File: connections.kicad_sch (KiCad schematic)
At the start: 27 parts, among them J1 Conn_01x04_Pin, J2 Conn_02x07_Odd_Even, J3 Conn_01x01_Pin, Q1 BSS138, Q2 BSS138

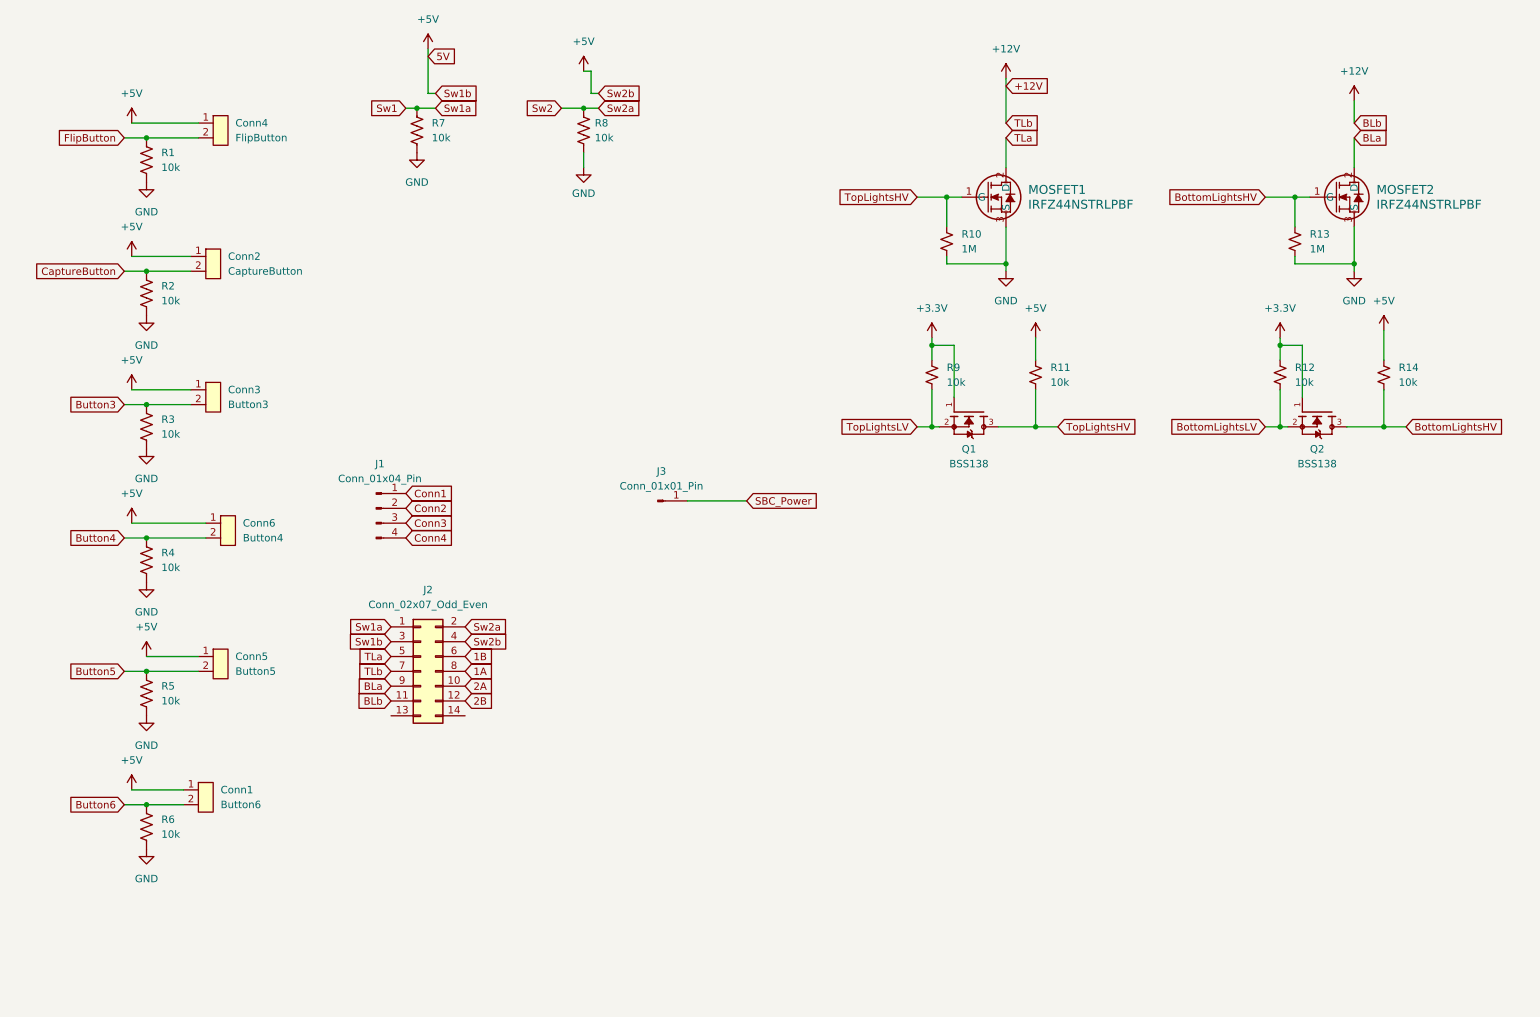
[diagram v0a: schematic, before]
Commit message: Layout changes
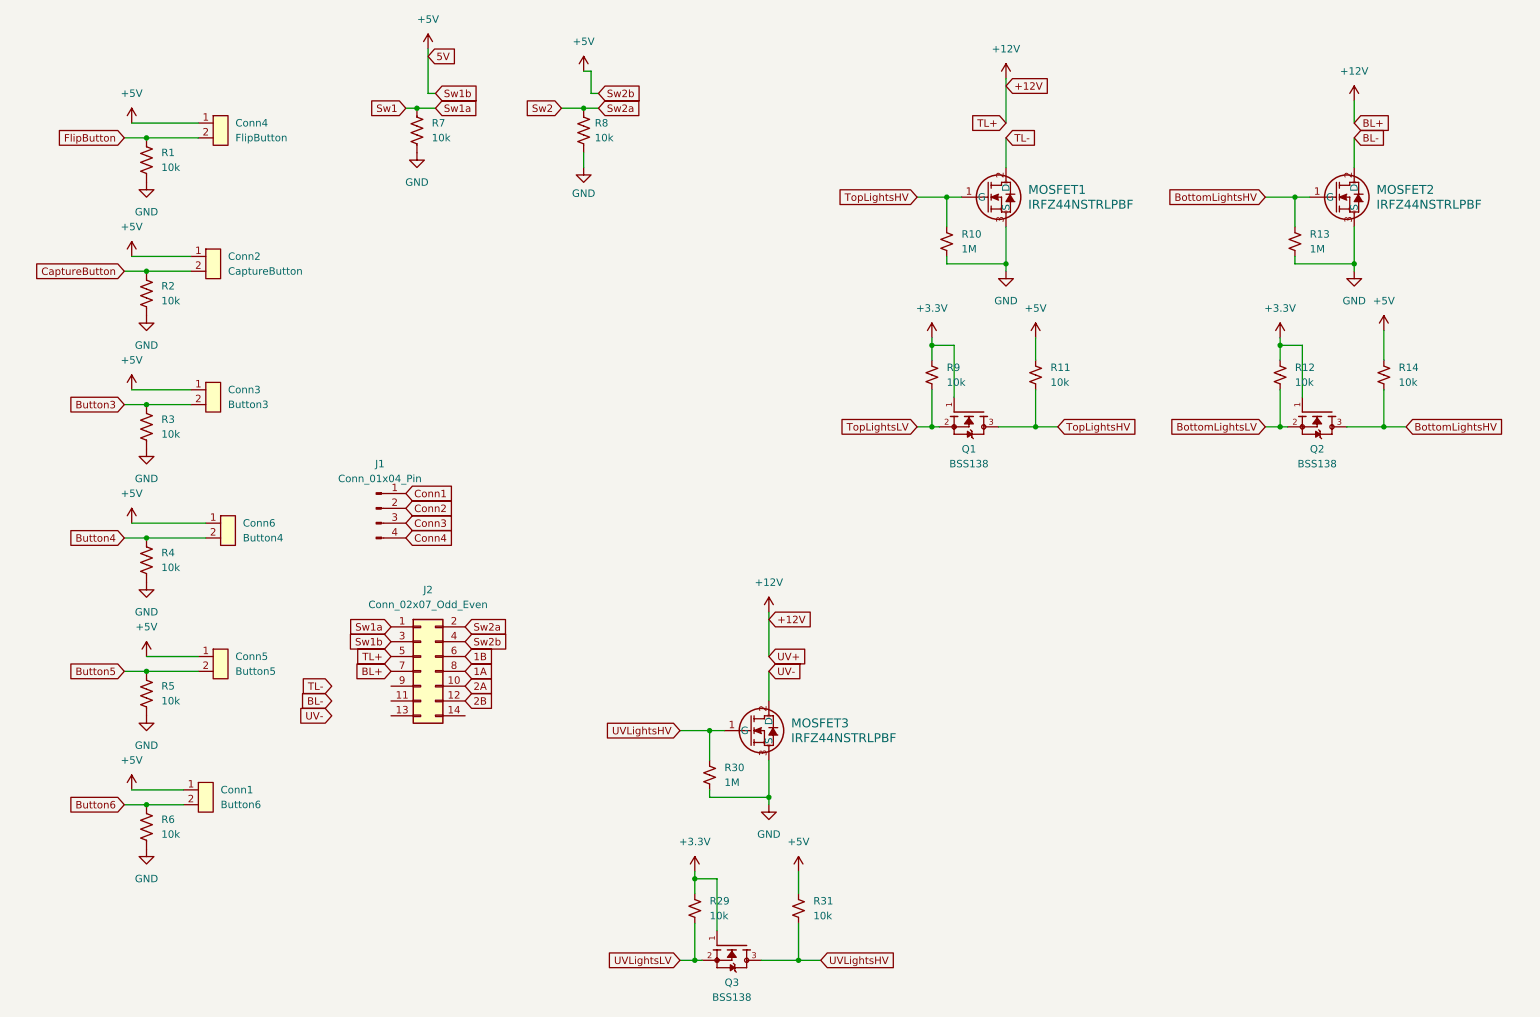
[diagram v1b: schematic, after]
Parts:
- removed J3: Conn_01x01_Pin, Connector_PinHeader_2.54mm:PinHeader_1x01_P2.54mm_Vertical, symbol Connector:Conn_01x01_Pin
- added MOSFET3: IRFZ44NSTRLPBF, IRFZ44NSTRLPBF:DPAK254P1524X483-3N, symbol 2024-05-21_14-07-33:IRFZ44NSTRLPBF
- added Q3: BSS138, BSS138:SOT95P240X111-3N, symbol BSS138:BSS138
- added R29, R31: 10k, Resistor_SMD:R_0603_1608Metric_Pad0.98x0.95mm_HandSolder, symbol Device:R_Small_US
- added R30: 1M, Resistor_SMD:R_0603_1608Metric_Pad0.98x0.95mm_HandSolder, symbol Device:R_Small_US
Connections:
- net +12V: now also J2.5 (Pin_5); no longer J2.11 (Pin_11)
- net +3.3V: now also Q3.1, R29.1
- net +5V: now also R31.1
- net GND: now also MOSFET3.3 (S), R30.2
- net BLa: no longer names the net of J2.9 (Pin_9)
- net BLa: no longer MOSFET2.2 (D)
- net TLa renamed TL-
- net TL-: no longer J2.5 (Pin_5)
- new net BL-: MOSFET2.2 (D)
- new net UV-: MOSFET3.2 (D)
- new net UVLightsHV: MOSFET3.1 (G), Q3.3, R30.1, R31.2
- new net UVLightsLV: Q3.2, R29.2
